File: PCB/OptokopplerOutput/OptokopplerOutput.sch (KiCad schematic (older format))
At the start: 16 parts, among them J1+1 Power, J1-1 Power, J2+1 I2C, J2-1 I2C, U1 PIC16F1503-IP

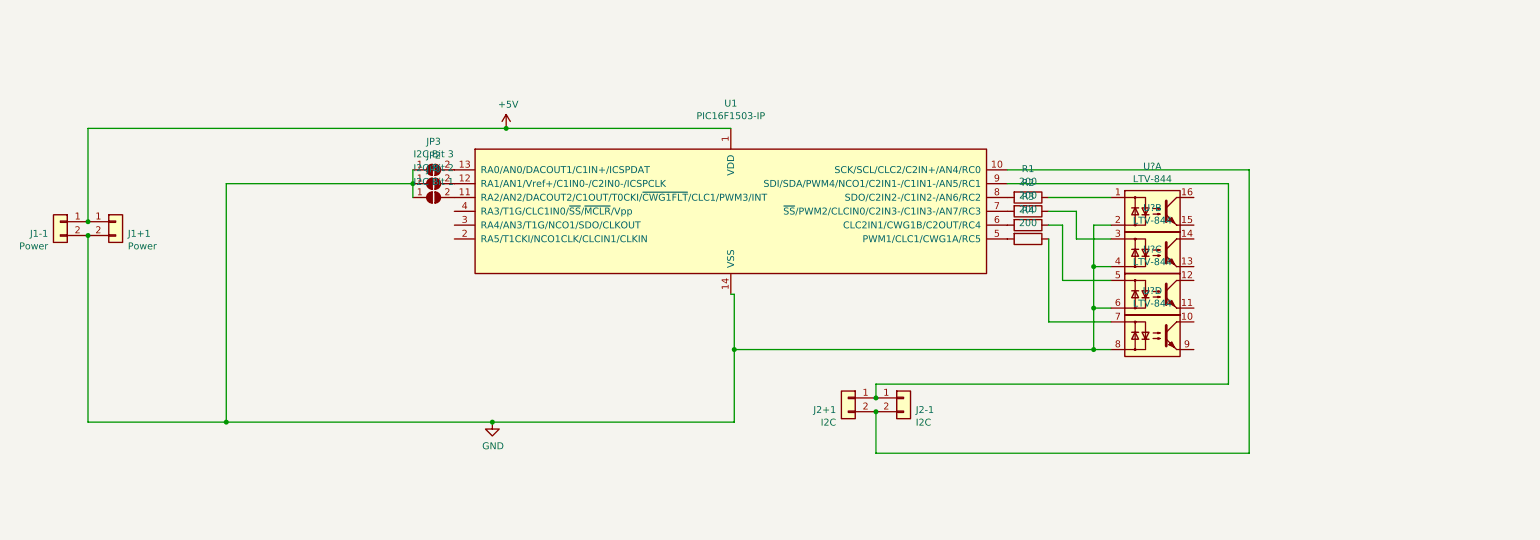
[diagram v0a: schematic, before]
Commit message: First try
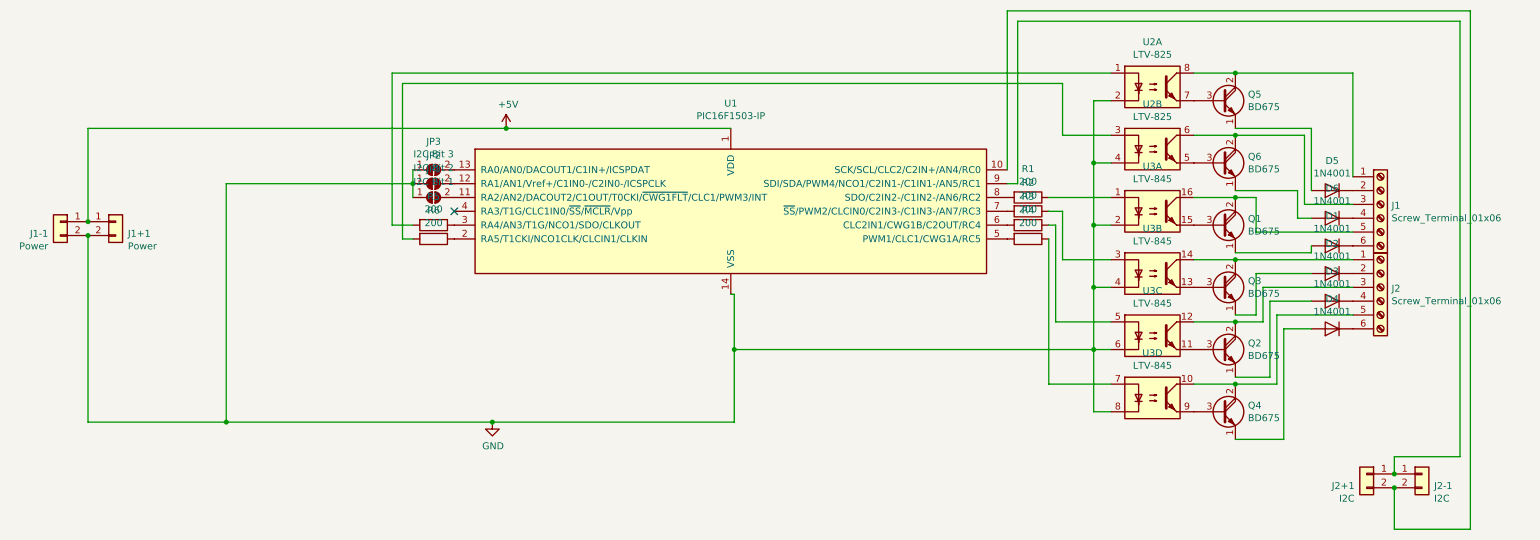
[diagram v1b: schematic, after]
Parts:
- removed U? (x4): LTV-844, Package_DIP:DIP-16_W7.62mm, symbol Isolator:LTV-844
- added D1, D2, D3, D4, D5, D6: 1N4001, Diode_SMD:D_SMB_Handsoldering, symbol Diode:1N4001
- added J1, J2: Screw_Terminal_01x06, TerminalBlock_RND:TerminalBlock_RND_205-00236_1x06_P5.08mm_Horizontal, symbol Connector:Screw_Terminal_01x06
- added Q1, Q2, Q3, Q4, Q5, Q6: BD675, Package_TO_SOT_THT:TO-126-3_Vertical, symbol Device:BD675
- added R5, R6: 200, Resistor_SMD:R_0603_1608Metric_Pad1.05x0.95mm_HandSolder, symbol Device:R
- added U2: LTV-825, Package_DIP:DIP-8_W7.62mm, symbol Isolator:LTV-825
- added U3: LTV-845, Package_DIP:DIP-16_W7.62mm, symbol Isolator:LTV-845
- R1, R2, R3, R4: footprint (none) -> Resistor_SMD:R_0603_1608Metric_Pad1.05x0.95mm_HandSolder
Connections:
- net GND: now also U2.2, U2.4, U3.2, U3.4, U3.6, U3.8
- net at U1.2 (RA5/T1CKI/NCO1CLK/CLCIN1/CLKIN): now also R6.1
- net at U1.3 (RA4/AN3/T1G/NCO1/SDO/CLKOUT): now also R5.1
- net at R1.1: now also U3.1
- net at R2.1: now also U3.3
- net at R3.1: now also U3.5
- net at R4.1: now also U3.7
- new net: D1.2 (A), Q1.1 (E)
- new net: J1.5 (Pin_5), Q1.2 (C), U3.16
- new net: Q1.3 (B), U3.15
- new net: D2.2 (A), Q3.1 (E)
- new net: J2.1 (Pin_1), Q3.2 (C), U3.14
- new net: Q3.3 (B), U3.13
- new net: D3.2 (A), Q2.1 (E)
- new net: J2.3 (Pin_3), Q2.2 (C), U3.12
- new net: Q2.3 (B), U3.11
- new net: D4.2 (A), Q4.1 (E)
- new net: J2.5 (Pin_5), Q4.2 (C), U3.10
- new net: Q4.3 (B), U3.9
- new net: D1.1 (K), J1.6 (Pin_6)
- new net: D2.1 (K), J2.2 (Pin_2)
- new net: D4.1 (K), J2.6 (Pin_6)
- new net: D3.1 (K), J2.4 (Pin_4)
- new net: J1.1 (Pin_1), Q5.2 (C), U2.8
- new net: D5.1 (K), J1.2 (Pin_2)
- new net: J1.3 (Pin_3), Q6.2 (C), U2.6
- new net: D6.1 (K), J1.4 (Pin_4)
- new net: R5.2, U2.1
- new net: Q5.3 (B), U2.7
- new net: R6.2, U2.3
- new net: Q6.3 (B), U2.5
- new net: D5.2 (A), Q5.1 (E)
- new net: D6.2 (A), Q6.1 (E)
- no-connect marks 0 -> 1
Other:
- moved on the sheet: J2+1, J2-1
